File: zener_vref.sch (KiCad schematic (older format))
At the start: 32 parts, among them J1 Conn_01x01, J2 Conn_01x01, J3 Conn_01x01, Q1 2SA733, Q2 2SC945, Q3 КТ639В, Q4 2SC945, Q5 2SC945

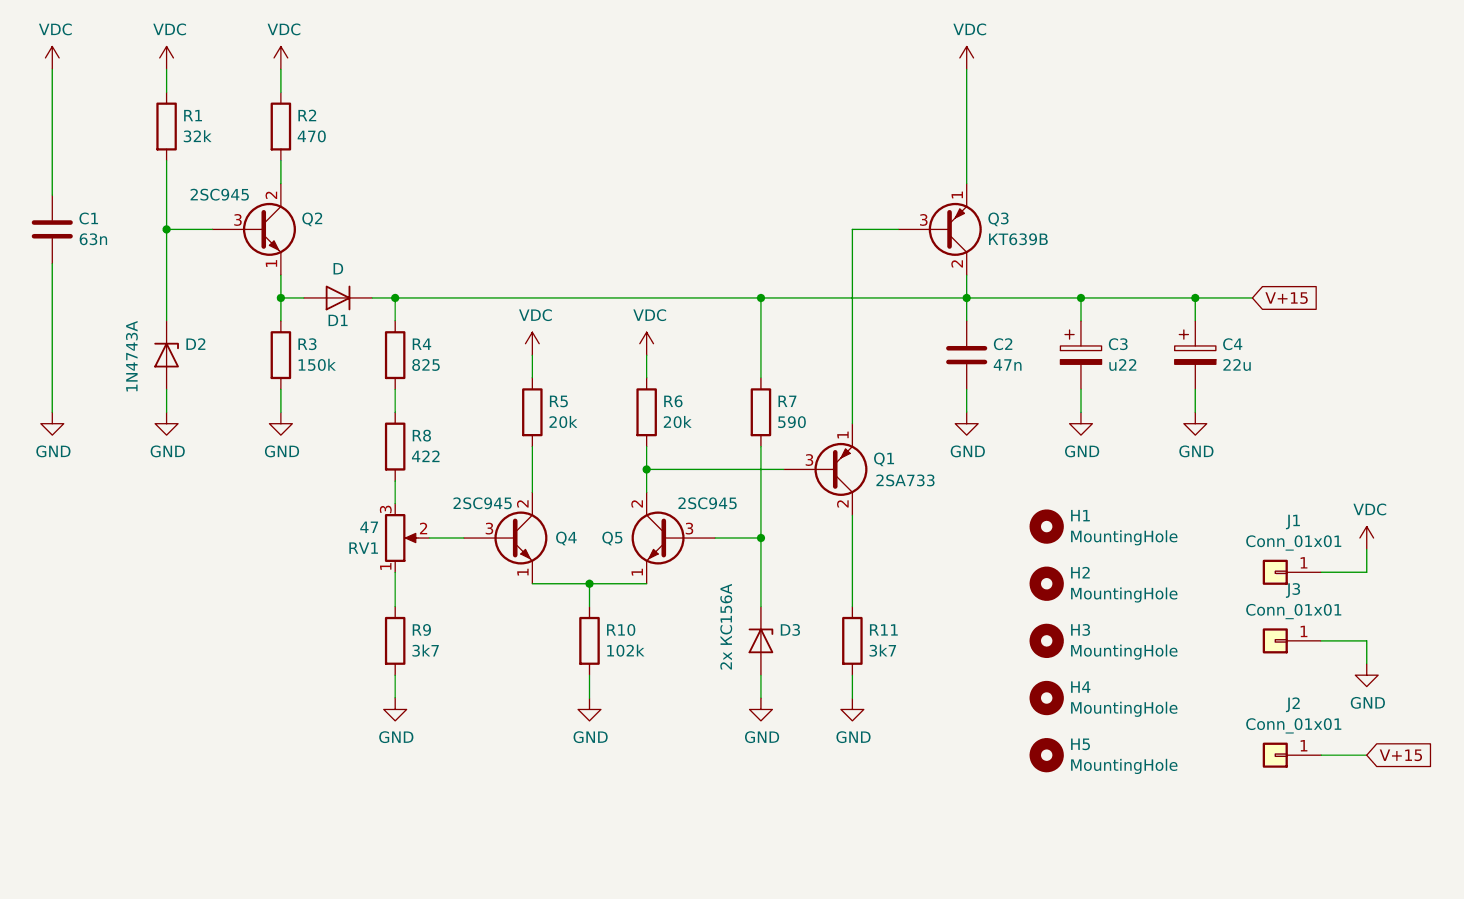
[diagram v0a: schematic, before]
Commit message: Version 1.3 : 10v KC156A
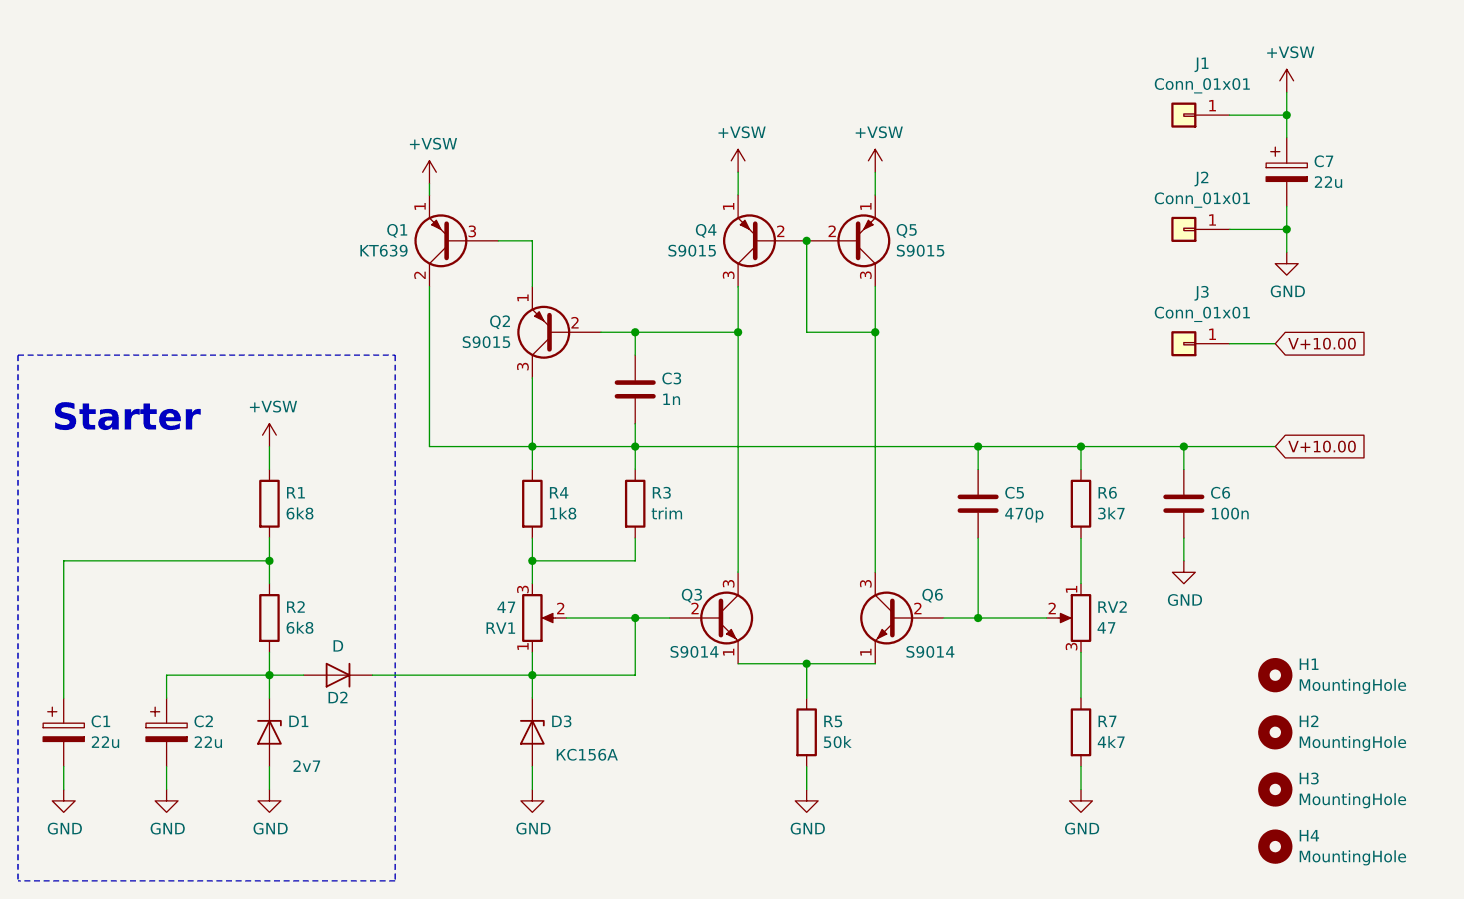
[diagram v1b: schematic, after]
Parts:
- removed C1: 63n, _сustom:LUT_C_Rect_L10.3mm_W5.0mm_P7.50mm, symbol Device:C
- removed C3: u22, _сustom:LUT_CP_Radial_D4.0mm_P2.00mm, symbol Device:CP
- removed C4: 22u, _сustom:LUT_CP_Radial_D5.0mm_P2.50mm, symbol Device:CP
- removed H5: MountingHole, MountingHole:MountingHole_2.7mm_M2.5, symbol Mechanical:MountingHole
- removed Q2, Q4, Q5: 2SC945, _сustom:LUT_TO-92, symbol Device:Q_NPN_ECB
- removed Q3: КТ639В, _сustom:LUT_TO-126-3_Vertical, symbol Device:Q_PNP_ECB
- removed R11: 3k7, _сustom:LUT_R_L9.0mm_D3.2mm_P12.70mm_Horizontal, symbol Device:R
- removed R3: 150k, _сustom:LUT_R_L9.0mm_D3.2mm_P12.70mm_Horizontal, symbol Device:R
- removed R5, R6: 20k, _сustom:LUT_R_L9.0mm_D3.2mm_P12.70mm_Horizontal, symbol Device:R
- removed R8: 422, _сustom:LUT_R_L9.0mm_D3.2mm_P12.70mm_Horizontal, symbol Device:R
- added C1, C2, C7: 22u, lut_foorprints:LUT_CP_Radial_D5.0mm_P2.50mm, symbol Device:CP
- added C3: 1n, lut_foorprints:LUT_C_Disc_D7.5mm_W2.5mm_P5.00mm, symbol Device:C
- added C5: 470p, lut_foorprints:LUT_C_Disc_D7.5mm_W2.5mm_P5.00mm, symbol Device:C
- added Q2, Q4, Q5: S9015, lut_foorprints:LUT_TO-92, symbol Device:Q_PNP_EBC
- added Q3, Q6: S9014, lut_foorprints:LUT_TO-92, symbol Device:Q_NPN_EBC
- added R4: 1k8, lut_foorprints:LUT_R_L9.9mm_D3.6mm_P12.70mm_Horizontal, symbol Device:R
- added RV1: 47, lut_foorprints:LUT_RPot_SP3-38B_Horizontal, symbol Device:R_POT
- C6: renamed from C2; value 47n -> 100n; footprint _сustom:LUT_C_Disc_D10.0mm_W2.5mm_P5.00mm -> lut_foorprints:LUT_C_Rect_L10.3mm_W5.0mm_P7.50mm
- D1: renamed from D2; value 1N4743A -> 2v7; footprint _сustom:LUT_D_P10.16mm_Horizontal -> lut_foorprints:LUT_D_P7.62mm_Horizontal
- D2: renamed from D1; footprint _сustom:LUT_D_P7.62mm_Horizontal -> lut_foorprints:LUT_D_P7.62mm_Horizontal
- D3: value 2x КС156А -> КС156А; footprint _сustom:LUT_D_P600_R-6_P7.62mm_Vertical_AnodeUp -> lut_foorprints:LUT_D_H7.0_W9.0_P30.48_Horizontal
- J1: footprint _сustom:LUT_PinHeader_1x01_P2.54mm_Vertical -> lut_foorprints:LUT_Wire_Clip_2_P2.54mm
- J2: renamed from J3; footprint _сustom:LUT_PinHeader_1x01_P2.54mm_Vertical -> lut_foorprints:LUT_Wire_Clip_2_P2.54mm
- J3: renamed from J2; footprint _сustom:LUT_PinHeader_1x01_P2.54mm_Vertical -> lut_foorprints:LUT_Wire_Clip_2_P2.54mm
- Q1: value 2SA733 -> KT639; footprint _сustom:LUT_TO-92 -> lut_foorprints:LUT_TO-126-3_Vertical
- R1: value 32k -> 6k8; footprint _сustom:LUT_R_L9.0mm_D3.2mm_P12.70mm_Horizontal -> lut_foorprints:LUT_R_L9.9mm_D3.6mm_P12.70mm_Horizontal
- R2: value 470 -> 6k8; footprint _сustom:LUT_R_L9.0mm_D3.2mm_P12.70mm_Horizontal -> lut_foorprints:LUT_R_L9.9mm_D3.6mm_P12.70mm_Horizontal
- R3: renamed from R4; value 825 -> trim; footprint _сustom:LUT_R_L9.0mm_D3.2mm_P12.70mm_Horizontal -> lut_foorprints:LUT_R_L9.9mm_D3.6mm_P12.70mm_Horizontal
- R5: renamed from R10; value 102k -> 50k; footprint _сustom:LUT_R_L9.0mm_D3.2mm_P12.70mm_Horizontal -> lut_foorprints:LUT_R_L9.9mm_D3.6mm_P12.70mm_Horizontal
- R6: renamed from R7; value 590 -> 3k7; footprint _сustom:LUT_R_L9.0mm_D3.2mm_P12.70mm_Horizontal -> lut_foorprints:LUT_R_L9.9mm_D3.6mm_P12.70mm_Horizontal
- R7: renamed from R9; value 3k7 -> 4k7; footprint _сustom:LUT_R_L9.0mm_D3.2mm_P12.70mm_Horizontal -> lut_foorprints:LUT_R_L9.9mm_D3.6mm_P12.70mm_Horizontal
- RV2: renamed from RV1; footprint _сustom:LUT_RPot_SP3-38B_Horizontal -> lut_foorprints:LUT_RPot_SP3-38B_Horizontal
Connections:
- net GND: now also C1.2, C2.2, C7.2
- net at R1.2: now also R2.1, C1.1; no longer D1.1 (K)
- net at R2.2: now also D1.1 (K), D2.2 (A), C2.1
- net at R3.2: now also R4.2, RV1.3
- net at RV2.3: now also R7.1
- net at RV2.1: now also R6.2; no longer R7.1
- net at RV2.2: now also C5.2, Q6.2 (B)
- net at D3.1 (K): now also D2.1 (K), Q3.2 (B), RV1.1, RV1.2; no longer R6.2
- net at R5.1: now also Q3.1 (E), Q6.1 (E)
- net at Q1.3 (B): now also Q2.1 (E)
- net +VSW: now reaches Q1.1 (E)
- net +VSW: now also J1.1 (Pin_1), R1.1, C7.1, Q4.1 (E), Q5.1 (E)
- net V+10.00: now reaches Q1.2 (C)
- net V+10.00: now also C6.1, J3.1 (Pin_1), R3.1, R6.1, C3.2, C5.1, Q2.3 (C), R4.1
- removed net V+15: C6.1, D2.1 (K), J3.1 (Pin_1), R3.1, R6.1
- removed net VDC: J1.1 (Pin_1), R1.1, R2.1
- new net: C3.1, Q2.2 (B), Q3.3 (C), Q4.3 (C)
- new net: Q4.2 (B), Q5.2 (B), Q5.3 (C), Q6.3 (C)
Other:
- note added: "Starter"
- moved on the sheet: C6, D1, D2, D3, H1, H2, H3, H4, J1, J2, J3, R1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
